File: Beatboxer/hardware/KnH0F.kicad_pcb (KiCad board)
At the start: 2 copper layers, 160 x 120 mm, 183 parts, among them J1 USB_C_Receptacle_USB2.0_16P, J2 Conn_01x06_Pin, SW1 SW_Push_45deg, SW10 SW_Push_45deg, SW11 SW_Push_45deg, SW12 SW_Push_45deg, SW13 SW_Push_45deg, SW14 SW_Push_45deg, SW15 SW_Push_45deg, SW16 SW_Push_45deg, SW17 SW_Push_45deg, SW18 SW_Push_45deg, SW19 SW_Push_45deg, SW2 SW_Push_45deg, SW20 SW_Push_45deg, SW21 SW_Push_45deg, SW22 SW_Push_45deg, SW23 SW_Push_45deg, SW24 SW_Push_45deg, SW25 SW_Push_45deg, SW26 SW_Push_45deg, SW27 SW_Push_45deg, SW28 SW_Push_45deg, SW29 SW_Push_45deg, SW3 SW_Push_45deg, SW30 SW_Push_45deg, SW31 SW_Push_45deg, SW32 SW_Push_45deg, SW33 SW_Push_45deg, SW34 SW_Push_45deg, SW35 SW_Push_45deg, SW36 SW_Push_45deg, SW37 SW_Push_45deg, SW38 SW_Push_45deg, SW39 SW_Push_45deg, SW4 SW_Push_45deg, SW40 SW_Push_45deg, SW41 SW_Push_45deg, SW42 SW_Push_45deg, SW43 SW_Push_45deg, SW44 SW_Push_45deg, SW45 SW_Push_45deg, SW46 SW_Push_45deg, SW47 SW_Push_45deg, SW48 SW_Push_45deg, SW49 SW_Push_45deg, SW5 SW_Push_45deg, SW50 SW_Push_45deg, SW51 SW_Push_45deg, SW52 SW_Push_45deg, SW53 SW_Push_45deg, SW54 SW_Push_45deg, SW55 SW_Push_45deg, SW56 SW_Push_45deg, SW57 SW_Push_45deg, SW58 SW_Push_45deg, SW59 SW_Push_45deg, SW6 SW_Push_45deg, SW60 SW_Push_45deg, SW61 SW_Push_45deg, SW62 SW_Push_45deg, SW63 SW_Push_45deg, SW64 SW_Push_45deg, SW65 SW_Push, SW66 SW_Push, SW67 SW_Push, SW7 SW_Push_45deg, SW8 SW_Push_45deg, SW9 SW_Push_45deg, U1 74AHC1G125, U2 AMS1117-3.3, U3 RP2040, U4 W25Q128JVS, Y1 12MHz

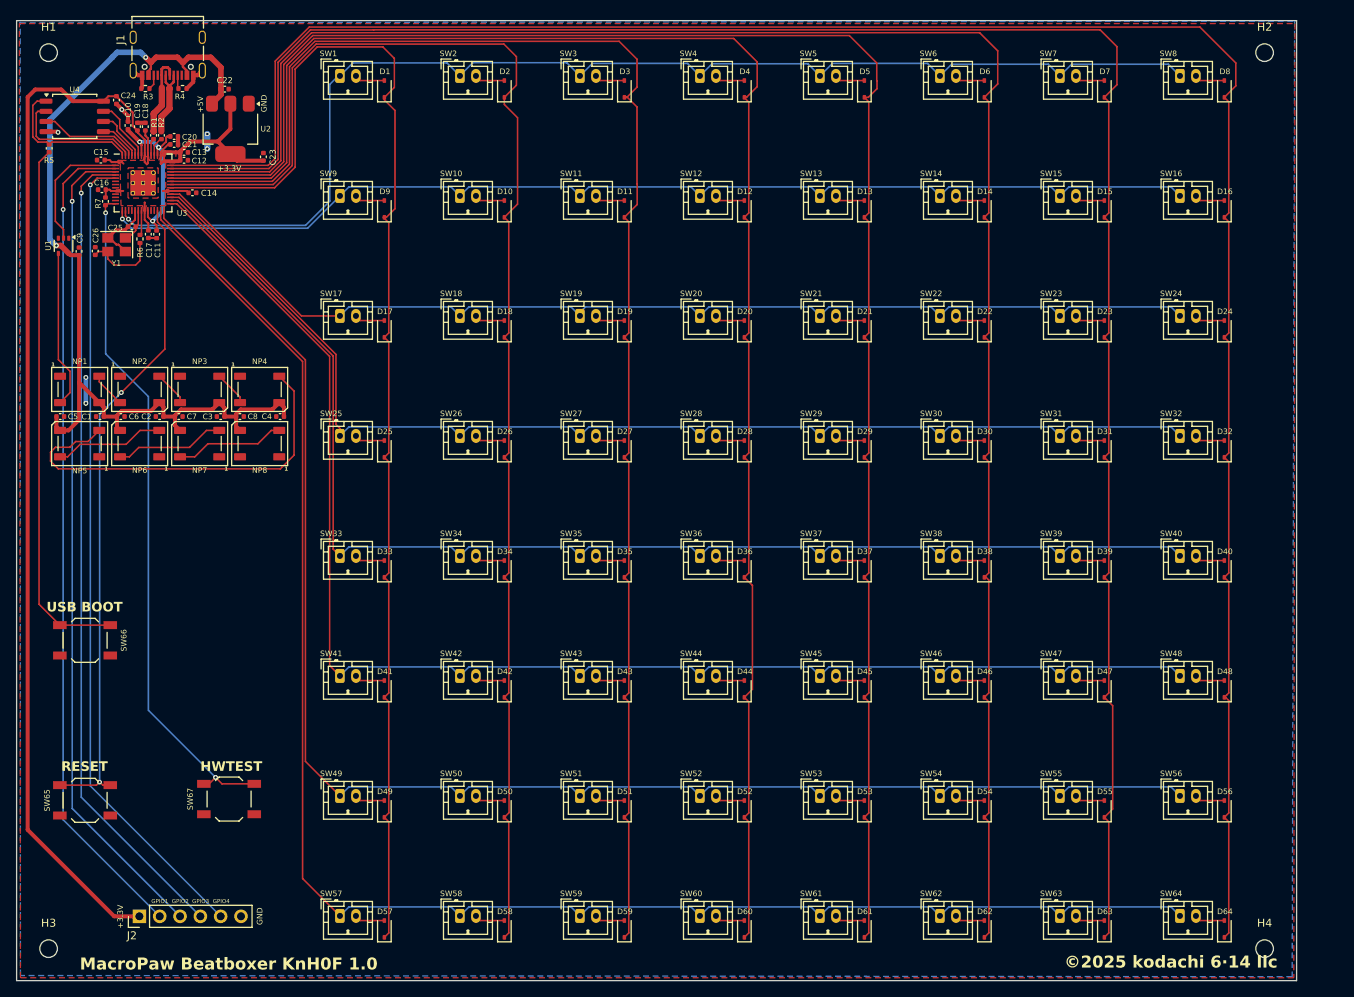
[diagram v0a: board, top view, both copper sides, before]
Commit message: BeatBoxer hardware as fabbed
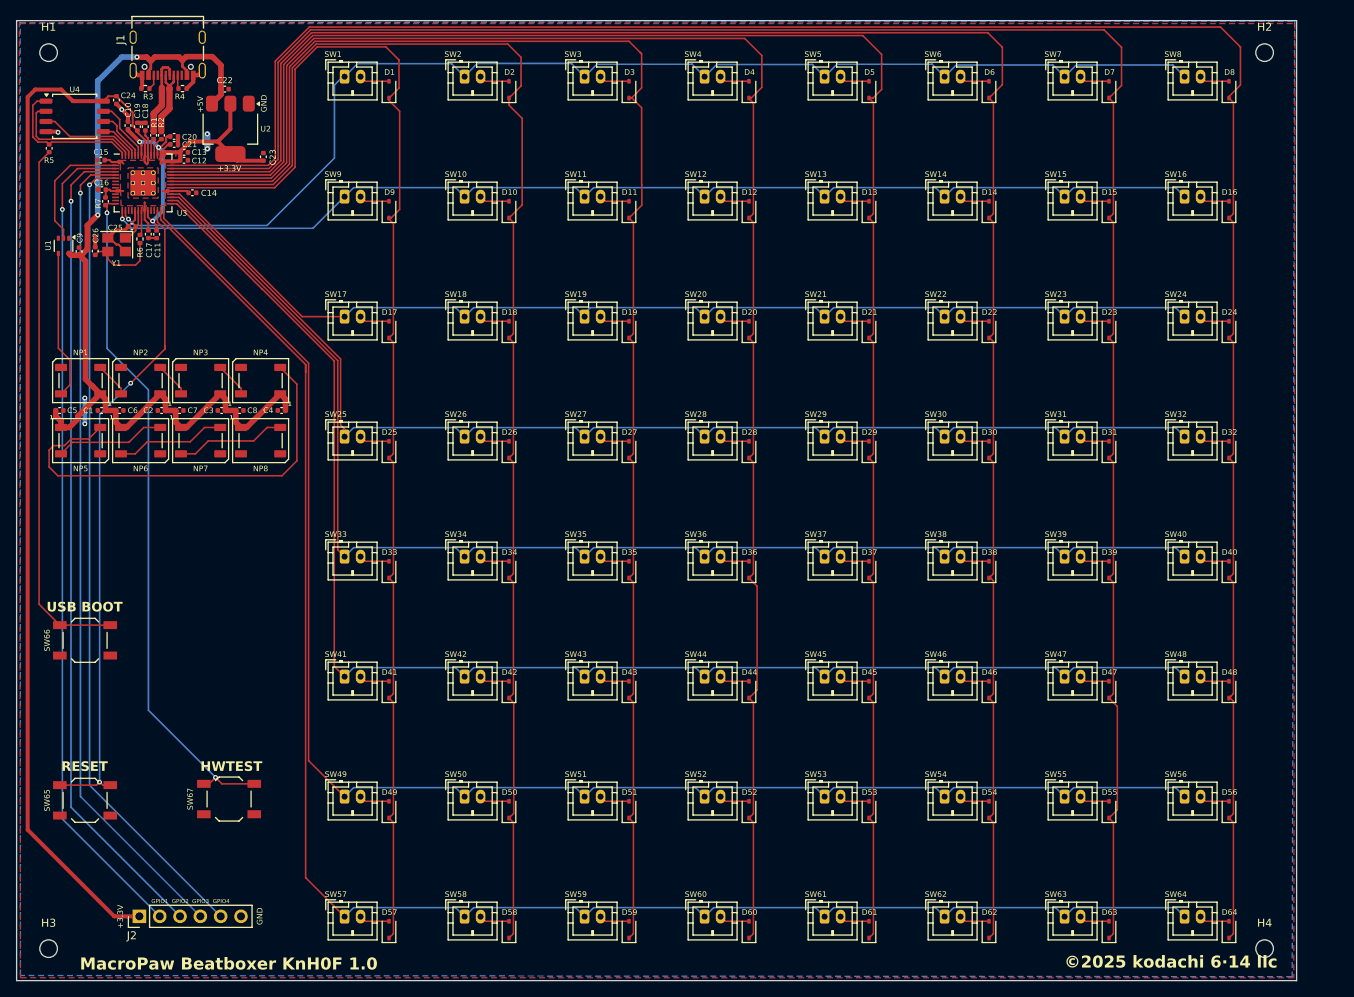
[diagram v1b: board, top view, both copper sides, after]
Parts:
- moved NP1 1.11 mm to (28.0, 65.0), turned to 180 degrees
- moved NP2 1.11 mm to (35.5, 65.0), turned to 180 degrees
- moved NP3 1.11 mm to (43.0, 65.0), turned to 180 degrees
- moved NP4 1.11 mm to (50.5, 65.0), turned to 180 degrees
- moved C2 0.80 mm to (38.1, 68.7)
- moved C1 0.79 mm to (30.6, 68.7)
- moved C4 0.78 mm to (53.1, 68.7)
- moved C6 0.77 mm to (32.9, 68.7)
- moved C3 0.77 mm to (45.6, 68.7)
- moved C7 0.77 mm to (40.4, 68.7)
- moved C5 0.76 mm to (25.4, 68.7)
- moved C8 0.76 mm to (47.9, 68.7)
- moved D30 0.59 mm to (141.6, 73.6)
- moved D31 0.59 mm to (156.6, 73.6)
- moved D32 0.59 mm to (171.6, 73.6)
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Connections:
- NP1 pad 1: GND -> +5V
- NP1 pad 2: /NEOPXL -> Net-(NP1-DOUT)
- NP1 pad 3: +5V -> GND
- NP1 pad 4: Net-(NP1-DOUT) -> /NEOPXL
- NP2 pad 1: GND -> +5V
- NP2 pad 2: Net-(NP1-DOUT) -> Net-(NP2-DOUT)
- NP2 pad 3: +5V -> GND
- NP2 pad 4: Net-(NP2-DOUT) -> Net-(NP1-DOUT)
- NP3 pad 1: GND -> +5V
- NP3 pad 2: Net-(NP2-DOUT) -> Net-(NP3-DOUT)
- NP3 pad 3: +5V -> GND
- NP3 pad 4: Net-(NP3-DOUT) -> Net-(NP2-DOUT)
- NP4 pad 1: GND -> +5V
- NP4 pad 2: Net-(NP3-DOUT) -> Net-(NP4-DOUT)
- NP4 pad 3: +5V -> GND
- NP4 pad 4: Net-(NP4-DOUT) -> Net-(NP3-DOUT)
- NP5 pad 1: GND -> +5V
- NP5 pad 2: Net-(NP4-DOUT) -> Net-(NP5-DOUT)
- NP5 pad 3: +5V -> GND
- NP5 pad 4: Net-(NP5-DOUT) -> Net-(NP4-DOUT)
- NP6 pad 1: GND -> +5V
- NP6 pad 2: Net-(NP5-DOUT) -> Net-(NP6-DOUT)
- NP6 pad 3: +5V -> GND
- NP6 pad 4: Net-(NP6-DOUT) -> Net-(NP5-DOUT)
- NP7 pad 1: GND -> +5V
- NP7 pad 2: Net-(NP6-DOUT) -> Net-(NP7-DOUT)
- NP7 pad 3: +5V -> GND
- NP7 pad 4: Net-(NP7-DOUT) -> Net-(NP6-DOUT)
- NP8 pad 1: GND -> +5V
- NP8 pad 2: Net-(NP7-DOUT) -> unconnected-(NP8-DOUT-Pad2)
- NP8 pad 3: +5V -> GND
- NP8 pad 4: unconnected-(NP8-DOUT-Pad4) -> Net-(NP7-DOUT)
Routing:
- net Net-(NP4-DOUT): track 50.5 -> 54.4 mm
- net ROW0: track 158.3 -> 155.6 mm
- net COL7: track 262.5 -> 264.1 mm
- net GND: track 27.2 -> 28.6 mm
- net COL4: track 217.5 -> 218.8 mm
- net COL2: track 188.5 -> 189.8 mm
- net ROW7: track 209.0 -> 210.2 mm
- net +5V: track 120.7 -> 119.4 mm
- net COL3: track 202.8 -> 203.9 mm
- net /NEOPXL: track 19.8 -> 18.6 mm
- net COL5: track 233.7 -> 234.6 mm
- net ROW2: track 139.9 -> 140.5 mm
- net COL1: track 173.2 -> 173.8 mm
- net COL6: track 249.1 -> 249.7 mm
- net /RUN: track 81.8 -> 82.4 mm
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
